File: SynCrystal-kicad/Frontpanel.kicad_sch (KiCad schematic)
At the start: 14 parts, among them SW1 Mode -, SW2 Mode +, SW3 Frame -, SW4 Frame +

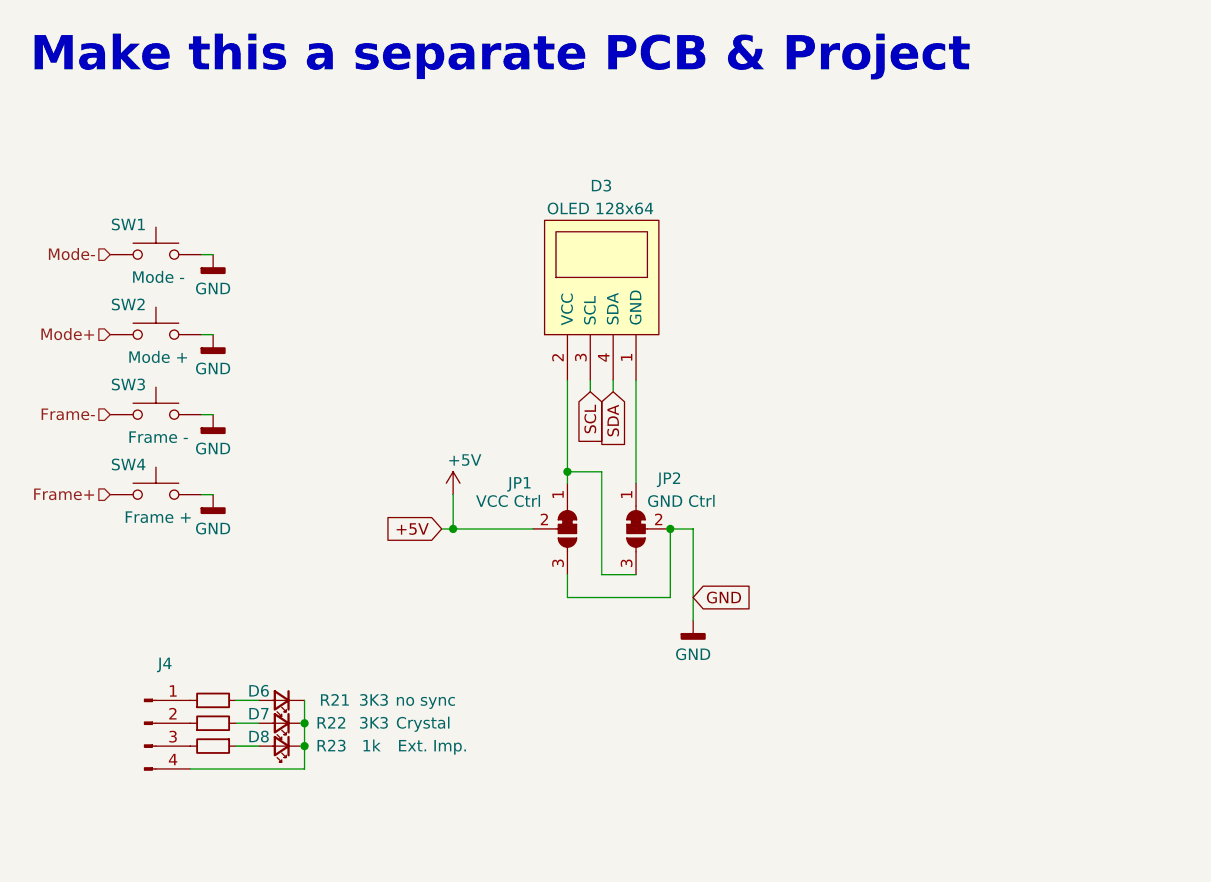
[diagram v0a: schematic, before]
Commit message: More changes
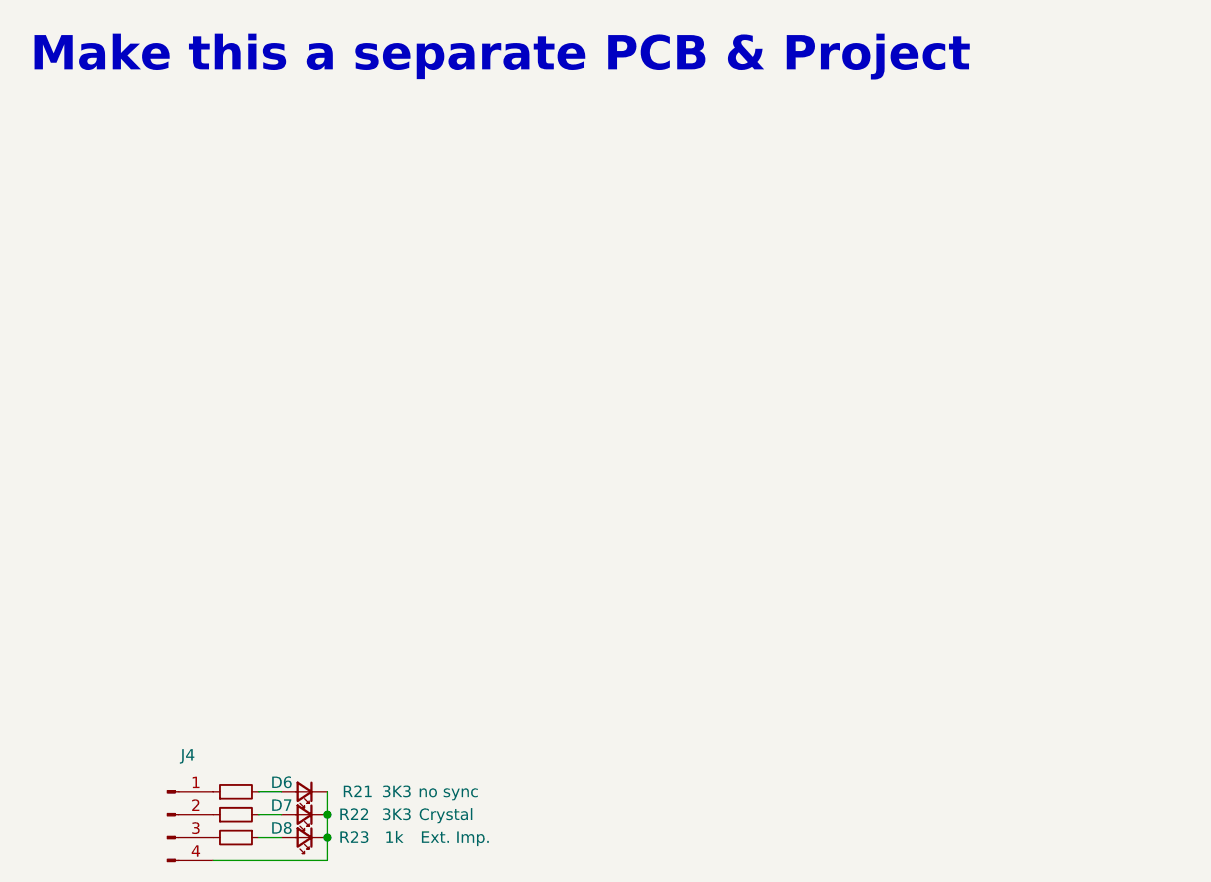
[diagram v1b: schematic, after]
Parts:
- removed D3: OLED 128x64, Peacemans Teile:OLED_128x63_i2c_0.96, symbol Peacemans Teile:OLED-128-64-I2C-Display_Character
- removed JP1: VCC Ctrl, Jumper:SolderJumper-3_P1.3mm_Bridged2Bar12_RoundedPad1.0x1.5mm, symbol Jumper:SolderJumper_3_Bridged12
- removed JP2: GND Ctrl, Jumper:SolderJumper-3_P1.3mm_Bridged2Bar12_RoundedPad1.0x1.5mm, symbol Jumper:SolderJumper_3_Bridged12
- removed SW1: Mode -, Button_Switch_SMD:SW_SPST_PTS647_Sx50, symbol Switch:SW_Push
- removed SW2: Mode +, Button_Switch_SMD:SW_SPST_PTS647_Sx50, symbol Switch:SW_Push
- removed SW3: Frame -, Button_Switch_SMD:SW_SPST_PTS647_Sx50, symbol Switch:SW_Push
- removed SW4: Frame +, Button_Switch_SMD:SW_SPST_PTS647_Sx50, symbol Switch:SW_Push
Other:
- moved on the sheet: D6, D7, D8, J4, R21, R22, R23
